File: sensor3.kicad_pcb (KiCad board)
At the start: 2 copper layers, 25 x 70 mm, 21 parts, among them CON1 AVR-ISP-6, CON2 DM3AT-SF-PEJM5, IC1 ATMEGA328P-A, P1 POWER, P2 RX/TX, P3 I2C, SW1 START/STOP, SW2 FORMAT, U1 AE-LPS331AP, U2 SL-MPU9150, X1 8MHz

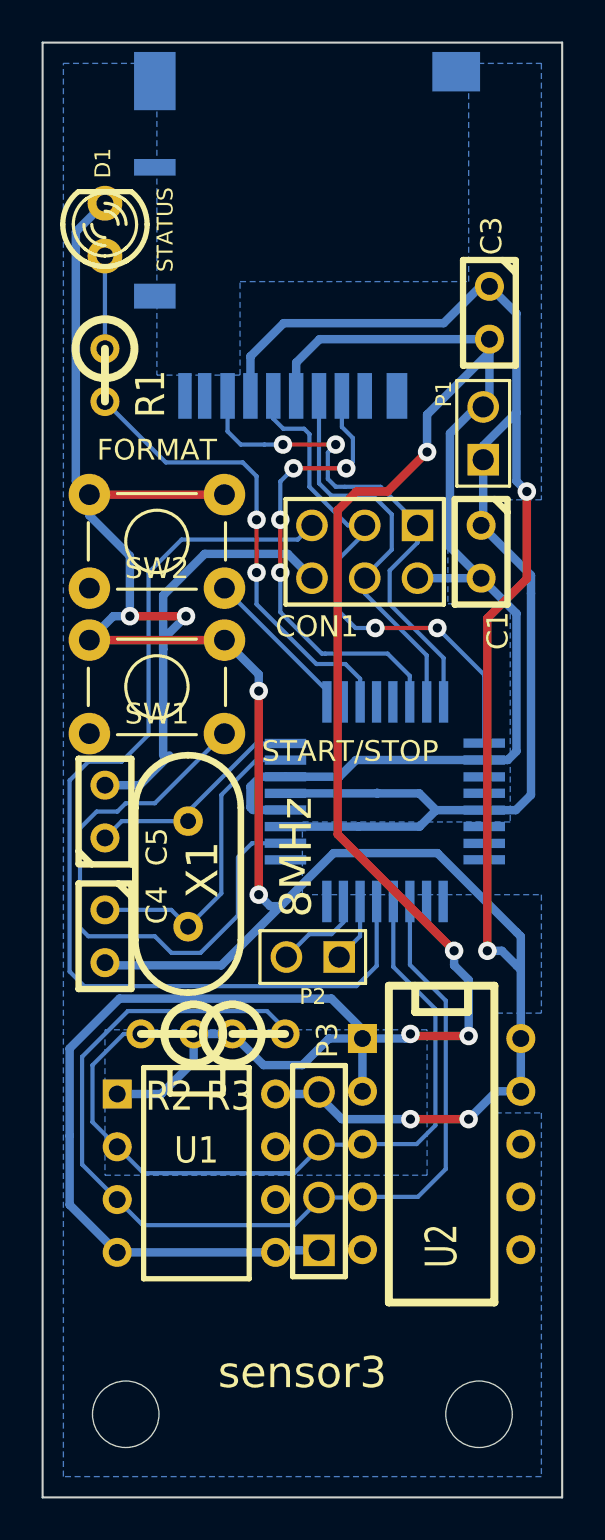
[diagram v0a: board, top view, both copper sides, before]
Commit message: Modify for halfside
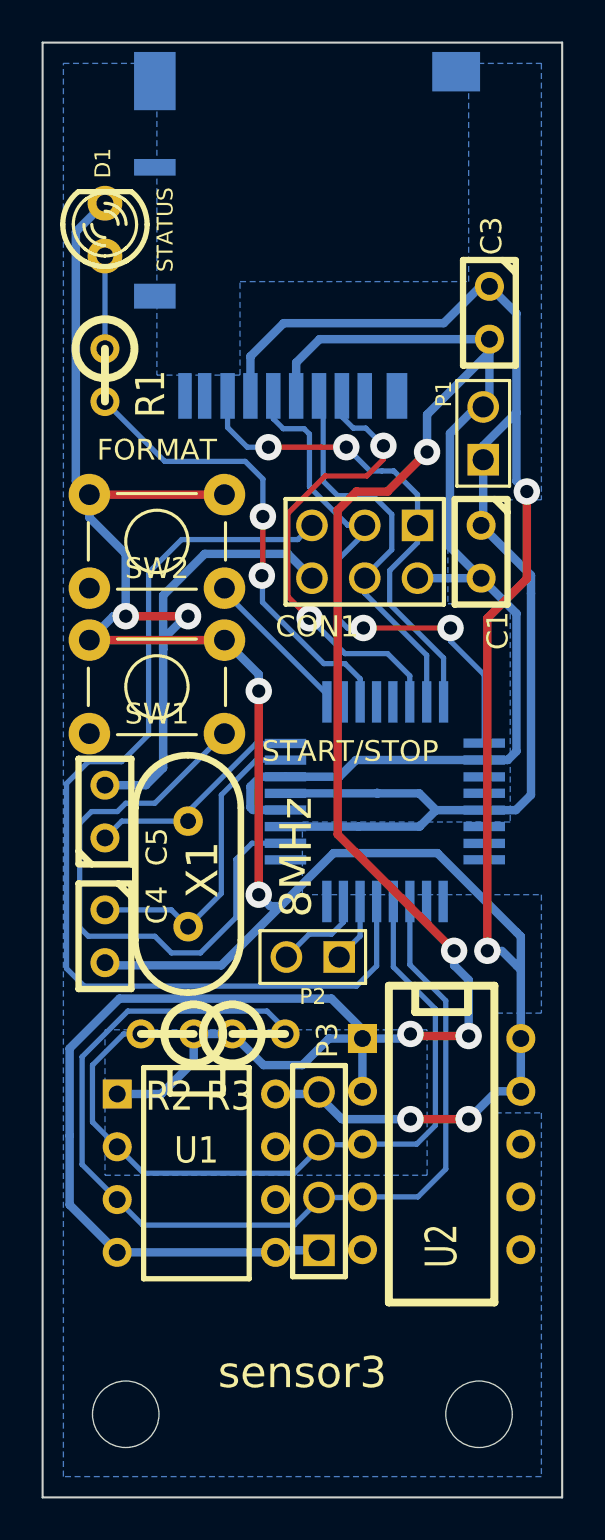
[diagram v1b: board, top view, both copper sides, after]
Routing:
- net N-0000040: track 24.4 -> 23.7 mm
- net N-0000041: track 25.8 -> 26.4 mm
- net N-0000010: track 22.5 -> 22.8 mm, vias 4 -> 2
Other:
- net class Bold: via_dia 0.889 -> 1.27
- net class Default: trace_width 0.2032 -> 0.254; via_dia 0.889 -> 1.27
